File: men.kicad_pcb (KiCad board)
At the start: 2 copper layers, 70 x 74 mm, 154 parts, among them J1 USB_C_Receptacle, J2 UART, P1 ICSPforPICKit, Q1 IRLML6402, Q2 IRLML6402, SW1 SW_Push, U1 CH340E, U2 PIC16(L)F18324, U3 24FC256, U4 TC118SS, U5 TLV61225

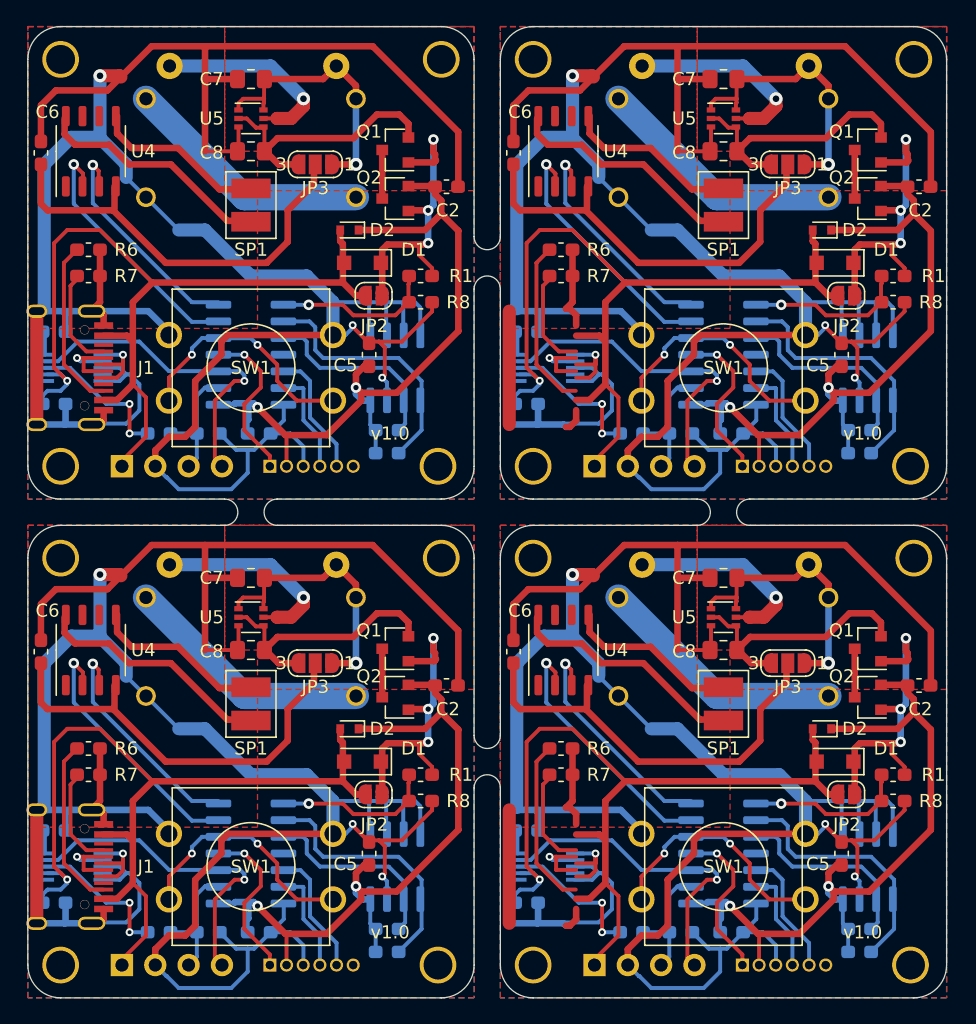
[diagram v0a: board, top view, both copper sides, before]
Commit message: ver2
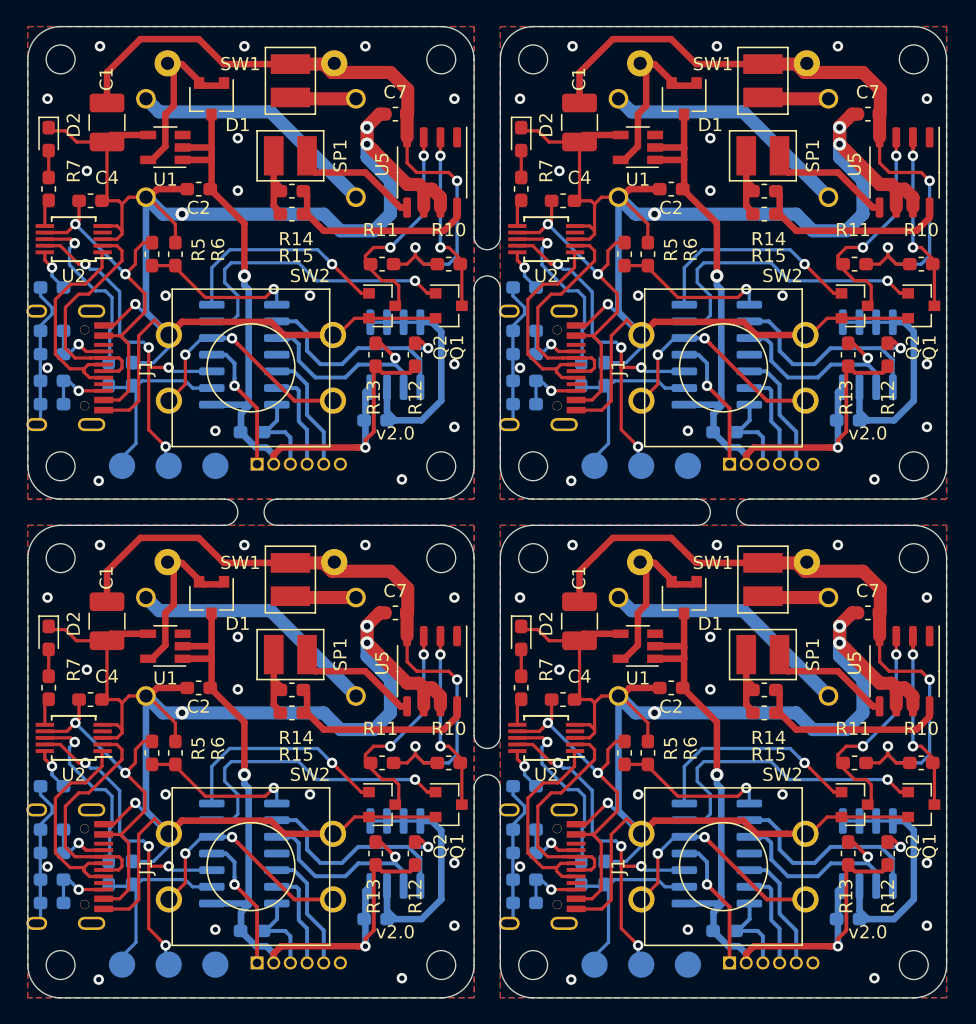
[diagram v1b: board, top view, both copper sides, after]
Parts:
- removed the BT1 at (65.0, 71.0)
- removed the BT1 at (29.0, 71.0)
- removed the BT1 at (65.0, 33.0)
- removed the BT1 at (29.0, 33.0)
- removed the BT2 at (81.0, 71.0)
- removed the BT2 at (45.0, 71.0)
- removed the BT2 at (81.0, 33.0)
- removed the BT2 at (45.0, 33.0)
- removed the C1 at (58.0, 81.2)
- removed the C1 at (22.0, 81.2)
- removed the C1 at (58.0, 43.2)
- removed the C1 at (22.0, 43.2)
- removed the C2 at (87.9, 70.2)
- removed the C2 at (51.9, 70.2)
- removed the C2 at (87.9, 32.2)
- removed the C2 at (51.9, 32.2)
- removed the C3 at (58.0, 86.8)
- removed the C3 at (22.0, 86.8)
- removed the C3 at (58.0, 48.8)
- removed the C3 at (22.0, 48.8)
- removed the C4 at (73.6, 89.0)
- removed the C4 at (37.6, 89.0)
- removed the C4 at (73.6, 51.0)
- removed the C4 at (37.6, 51.0)
- removed the C5 at (82.0, 83.0)
- removed the C5 at (46.0, 83.0)
- removed the C5 at (82.0, 45.0)
- removed the C5 at (46.0, 45.0)
- removed the C6 at (57.0, 67.6)
- removed the C6 at (21.0, 67.6)
- removed the C6 at (57.0, 29.6)
- removed the C6 at (21.0, 29.6)
- removed the C7 at (73.0, 62.0)
- removed the C7 at (37.0, 62.0)
- removed the C7 at (73.0, 24.0)
- removed the C7 at (37.0, 24.0)
- removed C8 (x4): C, Capacitor_SMD:C_0805_2012Metric_Pad1.15x1.40mm_HandSolder
- removed the D1 at (81.5, 76.0)
- removed the D1 at (45.5, 76.0)
- removed the D1 at (81.5, 38.0)
- removed the D1 at (45.5, 38.0)
- removed the D2 at (80.5, 73.5)
- removed the D2 at (44.5, 73.5)
- removed the D2 at (80.5, 35.5)
- removed the D2 at (44.5, 35.5)
- removed the H1 at (58.5, 60.5)
- removed the H1 at (22.5, 60.5)
- removed the H1 at (58.5, 22.5)
- removed the H1 at (22.5, 22.5)
- removed the H2 at (58.5, 91.5)
- removed the H2 at (22.5, 91.5)
- removed the H2 at (58.5, 53.5)
- removed the H2 at (22.5, 53.5)
- removed the H3 at (87.5, 60.5)
- removed the H3 at (51.5, 60.5)
- removed the H3 at (87.5, 22.5)
- removed the H3 at (51.5, 22.5)
- removed the H4 at (87.2, 91.5)
- removed the H4 at (51.2, 91.5)
- removed the H4 at (87.2, 53.5)
- removed the H4 at (51.2, 53.5)
- removed J2 (x4): UART, Connector_PinHeader_2.54mm:PinHeader_1x04_P2.54mm_Vertical
- removed JP2 (x4): D1_Bridge, Jumper:SolderJumper-2_P1.3mm_Open_RoundedPad1.0x1.5mm
- removed JP3 (x4): SP_SORCE, Jumper:SolderJumper-3_P1.3mm_Open_RoundedPad1.0x1.5mm_NumberLabels
- removed the L1 at (79.5, 61.0)
- removed the L1 at (43.5, 61.0)
- removed the L1 at (79.5, 23.0)
- removed the L1 at (43.5, 23.0)
- removed the P1 at (74.4, 91.5)
- removed the P1 at (38.4, 91.5)
- removed the P1 at (74.4, 53.5)
- removed the P1 at (38.4, 53.5)
- removed the Q1 at (84.0, 67.4)
- removed the Q1 at (48.0, 67.4)
- removed the Q1 at (84.0, 29.4)
- removed the Q1 at (48.0, 29.4)
- removed the Q2 at (84.0, 71.1)
- removed the Q2 at (48.0, 71.1)
- removed the Q2 at (84.0, 33.1)
- removed the Q2 at (48.0, 33.1)
- removed the R1 at (85.9, 77.0)
- removed the R1 at (49.9, 77.0)
- removed the R1 at (85.9, 39.0)
- removed the R1 at (49.9, 39.0)
- removed the R2 at (83.4, 90.5)
- removed the R2 at (47.4, 90.5)
- removed the R2 at (83.4, 52.5)
- removed the R2 at (47.4, 52.5)
- removed the R3 at (83.4, 88.8)
- removed the R3 at (47.4, 88.8)
- removed the R3 at (83.4, 50.8)
- removed the R3 at (47.4, 50.8)
- removed the R4 at (66.0, 89.0)
- removed the R4 at (30.0, 89.0)
- removed the R4 at (66.0, 51.0)
- removed the R4 at (30.0, 51.0)
- removed the R5 at (69.8, 89.0)
- removed the R5 at (33.8, 89.0)
- removed the R5 at (69.8, 51.0)
- removed the R5 at (33.8, 51.0)
- removed the R6 at (60.6, 75.0)
- removed the R6 at (24.6, 75.0)
- removed the R6 at (60.6, 37.0)
- removed the R6 at (24.6, 37.0)
- removed the R7 at (60.6, 77.0)
- removed the R7 at (24.6, 77.0)
- removed the R7 at (60.6, 39.0)
- removed the R7 at (24.6, 39.0)
- removed the R8 at (85.9, 79.0)
- removed the R8 at (49.9, 79.0)
- removed the R8 at (85.9, 41.0)
- removed the R8 at (49.9, 41.0)
- removed the SP1 at (73.0, 71.6)
- removed the SP1 at (37.0, 71.6)
- removed the SP1 at (73.0, 33.6)
- removed the SP1 at (37.0, 33.6)
- removed the SW1 at (73.0, 84.0)
- removed the SW1 at (37.0, 84.0)
- removed the SW1 at (73.0, 46.0)
- removed the SW1 at (37.0, 46.0)
- removed the U1 at (59.5, 84.0)
- removed the U1 at (23.5, 84.0)
- removed the U1 at (59.5, 46.0)
- removed the U1 at (23.5, 46.0)
- removed the U2 at (73.0, 83.0)
- removed the U2 at (37.0, 83.0)
- removed the U2 at (73.0, 45.0)
- removed the U2 at (37.0, 45.0)
- removed the U3 at (84.0, 84.0)
- removed the U3 at (48.0, 84.0)
- removed the U3 at (84.0, 46.0)
- removed the U3 at (48.0, 46.0)
- removed the U4 at (60.8, 67.5)
- removed the U4 at (24.8, 67.5)
- removed the U4 at (60.8, 29.5)
- removed the U4 at (24.8, 29.5)
- removed the U5 at (73.0, 65.0)
- removed the U5 at (37.0, 65.0)
- removed the U5 at (73.0, 27.0)
- removed the U5 at (37.0, 27.0)
- added BT1: Battery_Cell, fues-Battery_Holders:CH23-1225, B.Cu at (81.0, 71.0)
- added BT1: Battery_Cell, fues-Battery_Holders:CH23-1225, B.Cu at (45.0, 71.0)
- added BT1: Battery_Cell, fues-Battery_Holders:CH23-1225, B.Cu at (81.0, 33.0)
- added BT1: Battery_Cell, fues-Battery_Holders:CH23-1225, B.Cu at (45.0, 33.0)
- added BT2: Battery_Cell, fues-Battery_Holders:CH23-1225, B.Cu at (65.0, 71.0)
- added BT2: Battery_Cell, fues-Battery_Holders:CH23-1225, B.Cu at (29.0, 71.0)
- added BT2: Battery_Cell, fues-Battery_Holders:CH23-1225, B.Cu at (65.0, 33.0)
- added BT2: Battery_Cell, fues-Battery_Holders:CH23-1225, B.Cu at (29.0, 33.0)
- added C1: 47u, Capacitor_SMD:C_1210_3225Metric_Pad1.42x2.65mm_HandSolder, F.Cu at (62.0, 65.3)
- added C1: 47u, Capacitor_SMD:C_1210_3225Metric_Pad1.42x2.65mm_HandSolder, F.Cu at (26.0, 65.3)
- added C1: 47u, Capacitor_SMD:C_1210_3225Metric_Pad1.42x2.65mm_HandSolder, F.Cu at (62.0, 27.3)
- added C1: 47u, Capacitor_SMD:C_1210_3225Metric_Pad1.42x2.65mm_HandSolder, F.Cu at (26.0, 27.3)
- added C2: 22u, Capacitor_SMD:C_0603_1608Metric_Pad1.05x0.95mm_HandSolder, F.Cu at (69.0, 70.4)
- added C2: 22u, Capacitor_SMD:C_0603_1608Metric_Pad1.05x0.95mm_HandSolder, F.Cu at (33.0, 70.4)
- added C2: 22u, Capacitor_SMD:C_0603_1608Metric_Pad1.05x0.95mm_HandSolder, F.Cu at (69.0, 32.4)
- added C2: 22u, Capacitor_SMD:C_0603_1608Metric_Pad1.05x0.95mm_HandSolder, F.Cu at (33.0, 32.4)
- added C3: 0.1u 1608, Capacitor_SMD:C_0603_1608Metric_Pad1.05x0.95mm_HandSolder, B.Cu at (57.8, 77.9)
- added C3: 0.1u 1608, Capacitor_SMD:C_0603_1608Metric_Pad1.05x0.95mm_HandSolder, B.Cu at (21.8, 77.9)
- added C3: 0.1u 1608, Capacitor_SMD:C_0603_1608Metric_Pad1.05x0.95mm_HandSolder, B.Cu at (57.8, 39.9)
- added C3: 0.1u 1608, Capacitor_SMD:C_0603_1608Metric_Pad1.05x0.95mm_HandSolder, B.Cu at (21.8, 39.9)
- added C4: 0.1u 1608, Capacitor_SMD:C_0603_1608Metric_Pad1.05x0.95mm_HandSolder, F.Cu at (60.8, 71.3)
- added C4: 0.1u 1608, Capacitor_SMD:C_0603_1608Metric_Pad1.05x0.95mm_HandSolder, F.Cu at (24.8, 71.3)
- added C4: 0.1u 1608, Capacitor_SMD:C_0603_1608Metric_Pad1.05x0.95mm_HandSolder, F.Cu at (60.8, 33.3)
- added C4: 0.1u 1608, Capacitor_SMD:C_0603_1608Metric_Pad1.05x0.95mm_HandSolder, F.Cu at (24.8, 33.3)
- added C5: 0.1u 1608, Capacitor_SMD:C_0603_1608Metric_Pad1.05x0.95mm_HandSolder, B.Cu at (82.5, 88.0)
- added C5: 0.1u 1608, Capacitor_SMD:C_0603_1608Metric_Pad1.05x0.95mm_HandSolder, B.Cu at (46.5, 88.0)
- added C5: 0.1u 1608, Capacitor_SMD:C_0603_1608Metric_Pad1.05x0.95mm_HandSolder, B.Cu at (82.5, 50.0)
- added C5: 0.1u 1608, Capacitor_SMD:C_0603_1608Metric_Pad1.05x0.95mm_HandSolder, B.Cu at (46.5, 50.0)
- added C6: 0.1u 1608, Capacitor_SMD:C_0603_1608Metric_Pad1.05x0.95mm_HandSolder, B.Cu at (73.1, 88.9)
- added C6: 0.1u 1608, Capacitor_SMD:C_0603_1608Metric_Pad1.05x0.95mm_HandSolder, B.Cu at (37.1, 88.9)
- added C6: 0.1u 1608, Capacitor_SMD:C_0603_1608Metric_Pad1.05x0.95mm_HandSolder, B.Cu at (73.1, 50.9)
- added C6: 0.1u 1608, Capacitor_SMD:C_0603_1608Metric_Pad1.05x0.95mm_HandSolder, B.Cu at (37.1, 50.9)
- added C7: 0.1u 1608, Capacitor_SMD:C_0603_1608Metric_Pad1.05x0.95mm_HandSolder, F.Cu at (84.0, 64.7)
- added C7: 0.1u 1608, Capacitor_SMD:C_0603_1608Metric_Pad1.05x0.95mm_HandSolder, F.Cu at (48.0, 64.7)
- added C7: 0.1u 1608, Capacitor_SMD:C_0603_1608Metric_Pad1.05x0.95mm_HandSolder, F.Cu at (84.0, 26.7)
- added C7: 0.1u 1608, Capacitor_SMD:C_0603_1608Metric_Pad1.05x0.95mm_HandSolder, F.Cu at (48.0, 26.7)
- added D1: RB411D, Package_TO_SOT_SMD:SC-59, F.Cu at (70.0, 63.5)
- added D1: RB411D, Package_TO_SOT_SMD:SC-59, F.Cu at (34.0, 63.5)
- added D1: RB411D, Package_TO_SOT_SMD:SC-59, F.Cu at (70.0, 25.5)
- added D1: RB411D, Package_TO_SOT_SMD:SC-59, F.Cu at (34.0, 25.5)
- added D2: LED NC, Diode_SMD:D_0603_1608Metric_Pad1.05x0.95mm_HandSolder, F.Cu at (57.6, 66.6)
- added D2: LED NC, Diode_SMD:D_0603_1608Metric_Pad1.05x0.95mm_HandSolder, F.Cu at (21.6, 66.6)
- added D2: LED NC, Diode_SMD:D_0603_1608Metric_Pad1.05x0.95mm_HandSolder, F.Cu at (57.6, 28.6)
- added D2: LED NC, Diode_SMD:D_0603_1608Metric_Pad1.05x0.95mm_HandSolder, F.Cu at (21.6, 28.6)
- added H1: MountingHole, fues-mounting_hole:M2-drillHole_nosilk_nopad, F.Cu at (58.5, 60.5)
- added H1: MountingHole, fues-mounting_hole:M2-drillHole_nosilk_nopad, F.Cu at (22.5, 60.5)
- added H1: MountingHole, fues-mounting_hole:M2-drillHole_nosilk_nopad, F.Cu at (58.5, 22.5)
- added H1: MountingHole, fues-mounting_hole:M2-drillHole_nosilk_nopad, F.Cu at (22.5, 22.5)
- added H2: MountingHole, fues-mounting_hole:M2-drillHole_nosilk_nopad, F.Cu at (58.5, 91.5)
- added H2: MountingHole, fues-mounting_hole:M2-drillHole_nosilk_nopad, F.Cu at (22.5, 91.5)
- added H2: MountingHole, fues-mounting_hole:M2-drillHole_nosilk_nopad, F.Cu at (58.5, 53.5)
- added H2: MountingHole, fues-mounting_hole:M2-drillHole_nosilk_nopad, F.Cu at (22.5, 53.5)
- added H3: MountingHole, fues-mounting_hole:M2-drillHole_nosilk_nopad, F.Cu at (87.5, 60.5)
- added H3: MountingHole, fues-mounting_hole:M2-drillHole_nosilk_nopad, F.Cu at (51.5, 60.5)
- added H3: MountingHole, fues-mounting_hole:M2-drillHole_nosilk_nopad, F.Cu at (87.5, 22.5)
- added H3: MountingHole, fues-mounting_hole:M2-drillHole_nosilk_nopad, F.Cu at (51.5, 22.5)
- added H4: MountingHole, fues-mounting_hole:M2-drillHole_nosilk_nopad, F.Cu at (87.5, 91.5)
- added H4: MountingHole, fues-mounting_hole:M2-drillHole_nosilk_nopad, F.Cu at (51.5, 91.5)
- added H4: MountingHole, fues-mounting_hole:M2-drillHole_nosilk_nopad, F.Cu at (87.5, 53.5)
- added H4: MountingHole, fues-mounting_hole:M2-drillHole_nosilk_nopad, F.Cu at (51.5, 53.5)
- added J1: USB_C_Receptacle, fues-connect:USB_C_01, F.Cu at (62.5, 84.0)
- added J1: USB_C_Receptacle, fues-connect:USB_C_01, F.Cu at (62.5, 46.0)
- added L1: 100uH, Inductor_THT:L_Axial_L9.5mm_D4.0mm_P12.70mm_Horizontal_Fastron_SMCC, B.Cu at (79.3, 60.8)
- added L1: 100uH, Inductor_THT:L_Axial_L9.5mm_D4.0mm_P12.70mm_Horizontal_Fastron_SMCC, B.Cu at (43.4, 60.8)
- added L1: 100uH, Inductor_THT:L_Axial_L9.5mm_D4.0mm_P12.70mm_Horizontal_Fastron_SMCC, B.Cu at (79.3, 22.8)
- added L1: 100uH, Inductor_THT:L_Axial_L9.5mm_D4.0mm_P12.70mm_Horizontal_Fastron_SMCC, B.Cu at (43.4, 22.8)
- added P1: ICSPforPICKit, Connector_PinHeader_1.27mm:PinHeader_1x06_P1.27mm_Vertical, B.Cu at (73.5, 91.3)
- added P1: ICSPforPICKit, Connector_PinHeader_1.27mm:PinHeader_1x06_P1.27mm_Vertical, B.Cu at (37.5, 91.3)
- added P1: ICSPforPICKit, Connector_PinHeader_1.27mm:PinHeader_1x06_P1.27mm_Vertical, B.Cu at (73.5, 53.3)
- added P1: ICSPforPICKit, Connector_PinHeader_1.27mm:PinHeader_1x06_P1.27mm_Vertical, B.Cu at (37.5, 53.3)
- added Q1: 2n7002, Package_TO_SOT_SMD:SOT-23, F.Cu at (88.1, 79.3)
- added Q1: 2n7002, Package_TO_SOT_SMD:SOT-23, F.Cu at (52.1, 79.3)
- added Q1: 2n7002, Package_TO_SOT_SMD:SOT-23, F.Cu at (88.1, 41.3)
- added Q1: 2n7002, Package_TO_SOT_SMD:SOT-23, F.Cu at (52.1, 41.3)
- added Q2: 2n7002, Package_TO_SOT_SMD:SOT-23, F.Cu at (83.0, 79.3)
- added Q2: 2n7002, Package_TO_SOT_SMD:SOT-23, F.Cu at (47.0, 79.3)
- added Q2: 2n7002, Package_TO_SOT_SMD:SOT-23, F.Cu at (83.0, 41.3)
- added Q2: 2n7002, Package_TO_SOT_SMD:SOT-23, F.Cu at (47.0, 41.3)
- added R1: 10k, Resistor_SMD:R_0603_1608Metric_Pad1.05x0.95mm_HandSolder, B.Cu at (57.8, 86.8)
- added R1: 10k, Resistor_SMD:R_0603_1608Metric_Pad1.05x0.95mm_HandSolder, B.Cu at (21.8, 86.8)
- added R1: 10k, Resistor_SMD:R_0603_1608Metric_Pad1.05x0.95mm_HandSolder, B.Cu at (57.8, 48.8)
- added R1: 10k, Resistor_SMD:R_0603_1608Metric_Pad1.05x0.95mm_HandSolder, B.Cu at (21.8, 48.8)
- added R10: 10k, Resistor_SMD:R_0603_1608Metric_Pad1.05x0.95mm_HandSolder, F.Cu at (88.1, 76.1)
- added R10: 10k, Resistor_SMD:R_0603_1608Metric_Pad1.05x0.95mm_HandSolder, F.Cu at (52.1, 76.1)
- added R10: 10k, Resistor_SMD:R_0603_1608Metric_Pad1.05x0.95mm_HandSolder, F.Cu at (88.1, 38.1)
- added R10: 10k, Resistor_SMD:R_0603_1608Metric_Pad1.05x0.95mm_HandSolder, F.Cu at (52.1, 38.1)
- added R11: 10k, Resistor_SMD:R_0603_1608Metric_Pad1.05x0.95mm_HandSolder, F.Cu at (83.0, 76.1)
- added R11: 10k, Resistor_SMD:R_0603_1608Metric_Pad1.05x0.95mm_HandSolder, F.Cu at (47.0, 76.1)
- added R11: 10k, Resistor_SMD:R_0603_1608Metric_Pad1.05x0.95mm_HandSolder, F.Cu at (83.0, 38.1)
- added R11: 10k, Resistor_SMD:R_0603_1608Metric_Pad1.05x0.95mm_HandSolder, F.Cu at (47.0, 38.1)
- added R12: 10k, Resistor_SMD:R_0603_1608Metric_Pad1.05x0.95mm_HandSolder, F.Cu at (85.5, 83.0)
- added R12: 10k, Resistor_SMD:R_0603_1608Metric_Pad1.05x0.95mm_HandSolder, F.Cu at (49.5, 83.0)
- added R12: 10k, Resistor_SMD:R_0603_1608Metric_Pad1.05x0.95mm_HandSolder, F.Cu at (85.5, 45.0)
- added R12: 10k, Resistor_SMD:R_0603_1608Metric_Pad1.05x0.95mm_HandSolder, F.Cu at (49.5, 45.0)
- added R13: 10k, Resistor_SMD:R_0603_1608Metric_Pad1.05x0.95mm_HandSolder, F.Cu at (82.5, 83.0)
- added R13: 10k, Resistor_SMD:R_0603_1608Metric_Pad1.05x0.95mm_HandSolder, F.Cu at (46.5, 83.0)
- added R13: 10k, Resistor_SMD:R_0603_1608Metric_Pad1.05x0.95mm_HandSolder, F.Cu at (82.5, 45.0)
- added R13: 10k, Resistor_SMD:R_0603_1608Metric_Pad1.05x0.95mm_HandSolder, F.Cu at (46.5, 45.0)
- added R14: 47, Resistor_SMD:R_0603_1608Metric_Pad1.05x0.95mm_HandSolder, F.Cu at (76.1, 70.5)
- added R14: 47, Resistor_SMD:R_0603_1608Metric_Pad1.05x0.95mm_HandSolder, F.Cu at (40.1, 70.5)
- added R14: 47, Resistor_SMD:R_0603_1608Metric_Pad1.05x0.95mm_HandSolder, F.Cu at (76.1, 32.5)
- added R14: 47, Resistor_SMD:R_0603_1608Metric_Pad1.05x0.95mm_HandSolder, F.Cu at (40.1, 32.5)
- added R15: 47, Resistor_SMD:R_0603_1608Metric_Pad1.05x0.95mm_HandSolder, F.Cu at (76.1, 72.3)
- added R15: 47, Resistor_SMD:R_0603_1608Metric_Pad1.05x0.95mm_HandSolder, F.Cu at (40.1, 72.3)
- added R15: 47, Resistor_SMD:R_0603_1608Metric_Pad1.05x0.95mm_HandSolder, F.Cu at (76.1, 34.3)
- added R15: 47, Resistor_SMD:R_0603_1608Metric_Pad1.05x0.95mm_HandSolder, F.Cu at (40.1, 34.3)
- added R2: 10k, Resistor_SMD:R_0603_1608Metric_Pad1.05x0.95mm_HandSolder, B.Cu at (57.8, 85.0)
- added R2: 10k, Resistor_SMD:R_0603_1608Metric_Pad1.05x0.95mm_HandSolder, B.Cu at (21.8, 85.0)
- added R2: 10k, Resistor_SMD:R_0603_1608Metric_Pad1.05x0.95mm_HandSolder, B.Cu at (57.8, 47.0)
- added R2: 10k, Resistor_SMD:R_0603_1608Metric_Pad1.05x0.95mm_HandSolder, B.Cu at (21.8, 47.0)
- added R3: 10k, Resistor_SMD:R_0603_1608Metric_Pad1.05x0.95mm_HandSolder, B.Cu at (57.8, 83.0)
- added R3: 10k, Resistor_SMD:R_0603_1608Metric_Pad1.05x0.95mm_HandSolder, B.Cu at (21.8, 83.0)
- added R3: 10k, Resistor_SMD:R_0603_1608Metric_Pad1.05x0.95mm_HandSolder, B.Cu at (57.8, 45.0)
- added R3: 10k, Resistor_SMD:R_0603_1608Metric_Pad1.05x0.95mm_HandSolder, B.Cu at (21.8, 45.0)
- added R4: 10k, Resistor_SMD:R_0603_1608Metric_Pad1.05x0.95mm_HandSolder, B.Cu at (57.8, 81.2)
- added R4: 10k, Resistor_SMD:R_0603_1608Metric_Pad1.05x0.95mm_HandSolder, B.Cu at (21.8, 81.2)
- added R4: 10k, Resistor_SMD:R_0603_1608Metric_Pad1.05x0.95mm_HandSolder, B.Cu at (57.8, 43.2)
- added R4: 10k, Resistor_SMD:R_0603_1608Metric_Pad1.05x0.95mm_HandSolder, B.Cu at (21.8, 43.2)
- added R5: 10k, Resistor_SMD:R_0603_1608Metric_Pad1.05x0.95mm_HandSolder, F.Cu at (65.5, 75.3)
- added R5: 10k, Resistor_SMD:R_0603_1608Metric_Pad1.05x0.95mm_HandSolder, F.Cu at (29.5, 75.3)
- added R5: 10k, Resistor_SMD:R_0603_1608Metric_Pad1.05x0.95mm_HandSolder, F.Cu at (65.5, 37.3)
- added R5: 10k, Resistor_SMD:R_0603_1608Metric_Pad1.05x0.95mm_HandSolder, F.Cu at (29.5, 37.3)
- added R6: 10k, Resistor_SMD:R_0603_1608Metric_Pad1.05x0.95mm_HandSolder, F.Cu at (67.2, 75.3)
- added R6: 10k, Resistor_SMD:R_0603_1608Metric_Pad1.05x0.95mm_HandSolder, F.Cu at (31.2, 75.3)
- added R6: 10k, Resistor_SMD:R_0603_1608Metric_Pad1.05x0.95mm_HandSolder, F.Cu at (67.2, 37.3)
- added R6: 10k, Resistor_SMD:R_0603_1608Metric_Pad1.05x0.95mm_HandSolder, F.Cu at (31.2, 37.3)
- added R7: 470 NC, Resistor_SMD:R_0603_1608Metric_Pad1.05x0.95mm_HandSolder, F.Cu at (57.6, 70.4)
- added R7: 470 NC, Resistor_SMD:R_0603_1608Metric_Pad1.05x0.95mm_HandSolder, F.Cu at (21.6, 70.4)
- added R7: 470 NC, Resistor_SMD:R_0603_1608Metric_Pad1.05x0.95mm_HandSolder, F.Cu at (57.6, 32.4)
- added R7: 470 NC, Resistor_SMD:R_0603_1608Metric_Pad1.05x0.95mm_HandSolder, F.Cu at (21.6, 32.4)
- added R8: 10k, Resistor_SMD:R_0603_1608Metric_Pad1.05x0.95mm_HandSolder, B.Cu at (62.2, 84.5)
- added R8: 10k, Resistor_SMD:R_0603_1608Metric_Pad1.05x0.95mm_HandSolder, B.Cu at (26.2, 84.5)
- added R8: 10k, Resistor_SMD:R_0603_1608Metric_Pad1.05x0.95mm_HandSolder, B.Cu at (62.2, 46.5)
- added R8: 10k, Resistor_SMD:R_0603_1608Metric_Pad1.05x0.95mm_HandSolder, B.Cu at (26.2, 46.5)
- added R9: 10k, Resistor_SMD:R_0603_1608Metric_Pad1.05x0.95mm_HandSolder, B.Cu at (63.9, 84.5)
- added R9: 10k, Resistor_SMD:R_0603_1608Metric_Pad1.05x0.95mm_HandSolder, B.Cu at (27.9, 84.5)
- added R9: 10k, Resistor_SMD:R_0603_1608Metric_Pad1.05x0.95mm_HandSolder, B.Cu at (63.9, 46.5)
- added R9: 10k, Resistor_SMD:R_0603_1608Metric_Pad1.05x0.95mm_HandSolder, B.Cu at (27.9, 46.5)
- added SP1: sp, fues-connect:2.54-2pin-lay, F.Cu at (76.0, 67.8)
- added SP1: sp, fues-connect:2.54-2pin-lay, F.Cu at (40.0, 67.8)
- added SP1: sp, fues-connect:2.54-2pin-lay, F.Cu at (76.0, 29.8)
- added SP1: sp, fues-connect:2.54-2pin-lay, F.Cu at (40.0, 29.8)
- added SW1: POWER, fues-connect:2.54-2pin-lay, F.Cu at (76.0, 62.1)
- added SW1: POWER, fues-connect:2.54-2pin-lay, F.Cu at (40.0, 62.1)
- added SW1: POWER, fues-connect:2.54-2pin-lay, F.Cu at (76.0, 24.1)
- added SW1: POWER, fues-connect:2.54-2pin-lay, F.Cu at (40.0, 24.1)
- added SW2: SW_Push, fues-Buttons_Switches:TVGP01-G73BB, F.Cu at (73.0, 84.0)
- added SW2: SW_Push, fues-Buttons_Switches:TVGP01-G73BB, F.Cu at (37.0, 84.0)
- added SW2: SW_Push, fues-Buttons_Switches:TVGP01-G73BB, F.Cu at (73.0, 46.0)
- added SW2: SW_Push, fues-Buttons_Switches:TVGP01-G73BB, F.Cu at (37.0, 46.0)
- added TP1: tp_PC2MC, TestPoint:TestPoint_Pad_D2.0mm, B.Cu at (63.2, 91.5)
- added TP1: tp_PC2MC, TestPoint:TestPoint_Pad_D2.0mm, B.Cu at (27.2, 91.5)
- added TP1: tp_PC2MC, TestPoint:TestPoint_Pad_D2.0mm, B.Cu at (63.2, 53.5)
- added TP1: tp_PC2MC, TestPoint:TestPoint_Pad_D2.0mm, B.Cu at (27.2, 53.5)
- added TP2: tp_MC2PC, TestPoint:TestPoint_Pad_D2.0mm, B.Cu at (66.7, 91.5)
- added TP2: tp_MC2PC, TestPoint:TestPoint_Pad_D2.0mm, B.Cu at (30.7, 91.5)
- added TP2: tp_MC2PC, TestPoint:TestPoint_Pad_D2.0mm, B.Cu at (66.7, 53.5)
- added TP2: tp_MC2PC, TestPoint:TestPoint_Pad_D2.0mm, B.Cu at (30.7, 53.5)
- added TP3: tp_GND, TestPoint:TestPoint_Pad_D2.0mm, B.Cu at (70.3, 91.5)
- added TP3: tp_GND, TestPoint:TestPoint_Pad_D2.0mm, B.Cu at (34.3, 91.5)
- added TP3: tp_GND, TestPoint:TestPoint_Pad_D2.0mm, B.Cu at (70.3, 53.5)
- added TP3: tp_GND, TestPoint:TestPoint_Pad_D2.0mm, B.Cu at (34.3, 53.5)
- added U1: HT77XXA_SOT-25, Package_TO_SOT_SMD:TSOT-23-5, F.Cu at (66.5, 67.2)
- added U1: HT77XXA_SOT-25, Package_TO_SOT_SMD:TSOT-23-5, F.Cu at (30.5, 67.2)
- added U1: HT77XXA_SOT-25, Package_TO_SOT_SMD:TSOT-23-5, F.Cu at (66.5, 29.2)
- added U1: HT77XXA_SOT-25, Package_TO_SOT_SMD:TSOT-23-5, F.Cu at (30.5, 29.2)
- added U2: CH340E, Package_SO:MSOP-10_3x3mm_P0.5mm, F.Cu at (59.5, 74.2)
- added U2: CH340E, Package_SO:MSOP-10_3x3mm_P0.5mm, F.Cu at (23.5, 74.2)
- added U2: CH340E, Package_SO:MSOP-10_3x3mm_P0.5mm, F.Cu at (59.5, 36.2)
- added U2: CH340E, Package_SO:MSOP-10_3x3mm_P0.5mm, F.Cu at (23.5, 36.2)
- added U3: PIC16(L)F18324, Package_SO:SOIC-14_3.9x8.7mm_P1.27mm, B.Cu at (72.5, 83.0)
- added U3: PIC16(L)F18324, Package_SO:SOIC-14_3.9x8.7mm_P1.27mm, B.Cu at (36.5, 83.0)
- added U3: PIC16(L)F18324, Package_SO:SOIC-14_3.9x8.7mm_P1.27mm, B.Cu at (72.5, 45.0)
- added U3: PIC16(L)F18324, Package_SO:SOIC-14_3.9x8.7mm_P1.27mm, B.Cu at (36.5, 45.0)
- added U4: 24FC256, Package_SO:SOIC-8_3.9x4.9mm_P1.27mm, B.Cu at (84.0, 83.0)
- added U4: 24FC256, Package_SO:SOIC-8_3.9x4.9mm_P1.27mm, B.Cu at (48.0, 83.0)
- added U4: 24FC256, Package_SO:SOIC-8_3.9x4.9mm_P1.27mm, B.Cu at (84.0, 45.0)
- added U4: 24FC256, Package_SO:SOIC-8_3.9x4.9mm_P1.27mm, B.Cu at (48.0, 45.0)
- added U5: TC118SS, Package_SO:SSOP-8_3.9x5.05mm_P1.27mm, F.Cu at (86.8, 69.1)
- added U5: TC118SS, Package_SO:SSOP-8_3.9x5.05mm_P1.27mm, F.Cu at (50.8, 69.1)
- added U5: TC118SS, Package_SO:SSOP-8_3.9x5.05mm_P1.27mm, F.Cu at (86.8, 31.1)
- added U5: TC118SS, Package_SO:SSOP-8_3.9x5.05mm_P1.27mm, F.Cu at (50.8, 31.1)
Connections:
- J1 pad A1: GND -> (no net)
- J1 pad A4: +5V -> (no net)
- J1 pad A5: Net-(J1-PadA5) -> (no net)
- J1 pad A6: /D+ -> (no net)
- J1 pad A7: /D- -> (no net)
- J1 pad A8: Net-(J1-PadA8) -> (no net)
- J1 pad B5: Net-(J1-PadB5) -> (no net)
- J1 pad B6: /D+ -> (no net)
- J1 pad B7: /D- -> (no net)
- J1 pad B8: Net-(J1-PadB8) -> (no net)
- J1 pad S1: GND -> (no net)
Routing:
- net (no net): track 2207.3 -> 2527.2 mm, vias 66 -> 184
- net GND: track 227.7 -> 0.00 mm, vias 3 -> 0
- net +5V: track 66.9 -> 0.00 mm, vias 1 -> 0
- net VDD: track 60.9 -> 0.00 mm, vias 2 -> 0
- net Net-(C6-Pad1): track 32.9 -> 0.00 mm
- net /UART_MC2PC: track 25.4 -> 0.00 mm, vias 1 -> 0
- net Net-(D1-Pad1): track 23.3 -> 0.00 mm, vias 3 -> 0
- net +BATT: track 20.8 -> 0.00 mm, vias 1 -> 0
- net +3V3: track 20.3 -> 0.00 mm
- net /SPD1: track 19.7 -> 0.00 mm, vias 1 -> 0
- net /SDA: track 19.7 -> 0.00 mm
- net Net-(BT1-Pad1): track 19.1 -> 0.00 mm
- net /SW: track 18.5 -> 0.00 mm, vias 2 -> 0
- net Net-(SP1-Pad1): track 18.3 -> 0.00 mm
- net /SPD2: track 17.4 -> 0.00 mm, vias 1 -> 0
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- removed copper zone on F.Cu, net +BATT
- removed copper zone on B.Cu, net GND
- removed copper zone on F.Cu, net GND
- removed copper zone on F.Cu, net VDD
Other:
- board text added: "kamibushiele.net"
- board text added: "v2.0"
- board text removed: "v1.0"
